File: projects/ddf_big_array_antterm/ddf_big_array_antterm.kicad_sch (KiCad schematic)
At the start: 11 parts, among them J1 Conn_Coaxial, J2 Conn_Coaxial

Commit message: release candidate
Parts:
- H1, H2, H3: now left out of the parts list
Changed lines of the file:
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@@
   )
   (symbol (lib_id "Mechanical:MountingHole_Pad") (at 48.006 170.434 0) (unit 1)
-    (in_bom yes) (on_board yes)
+    (in_bom no) (on_board yes)
     (property "Reference" "H1" (id 0) (at 50.546 169.1639 0)
       (effects (font (size 1.27 1.27)) (justify left))
@@
   )
   (symbol (lib_id "Mechanical:MountingHole_Pad") (at 65.151 170.434 0) (unit 1)
-    (in_bom yes) (on_board yes) (fields_autoplaced)
+    (in_bom no) (on_board yes) (fields_autoplaced)
     (property "Reference" "H2" (id 0) (at 67.691 169.1639 0)
       (effects (font (size 1.27 1.27)) (justify left))
@@
   )
   (symbol (lib_id "Mechanical:MountingHole_Pad") (at 82.296 170.434 0) (unit 1)
-    (in_bom yes) (on_board yes) (fields_autoplaced)
+    (in_bom no) (on_board yes) (fields_autoplaced)
     (property "Reference" "H3" (id 0) (at 84.836 169.1639 0)
       (effects (font (size 1.27 1.27)) (justify left))

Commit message: release candidate
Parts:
- H4: now left out of the parts list
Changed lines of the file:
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@@
   )
   (symbol (lib_id "Mechanical:MountingHole_Pad") (at 99.314 170.434 0) (unit 1)
-    (in_bom yes) (on_board yes) (fields_autoplaced)
+    (in_bom no) (on_board yes) (fields_autoplaced)
     (property "Reference" "H4" (id 0) (at 101.854 169.1639 0)
       (effects (font (size 1.27 1.27)) (justify left))

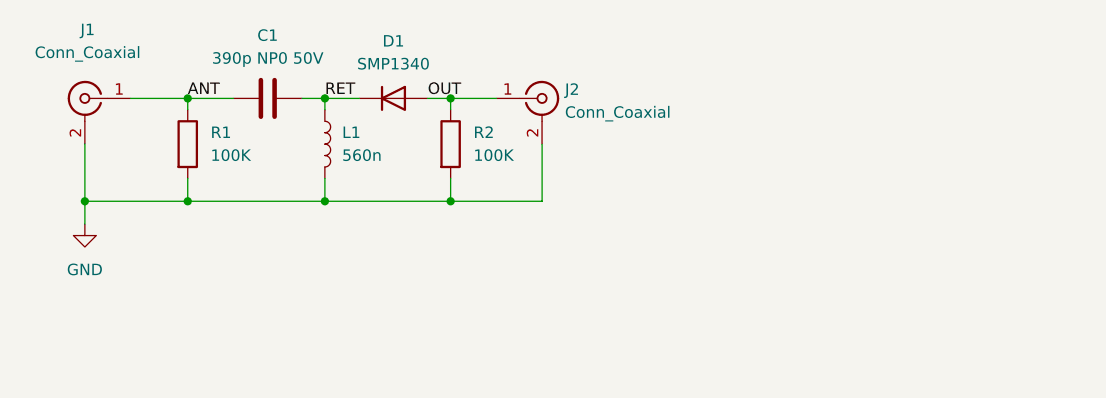
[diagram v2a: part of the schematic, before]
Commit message: release candidate
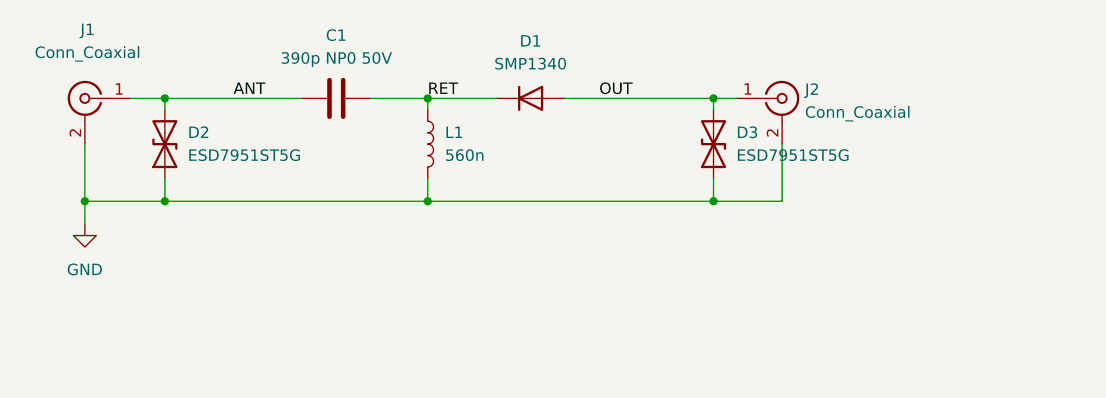
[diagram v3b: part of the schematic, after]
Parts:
- removed R1, R2: 100K, Resistor_SMD:R_0603_1608Metric, symbol Device:R
- added D2, D3: ESD7951ST5G, Diode_SMD:D_SOD-923, symbol Device:D_TVS
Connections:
- net ANT: now also D2.2 (A2)
- net GND: now also D2.1 (A1), D3.1 (A1)
- net OUT: now also D3.2 (A2)
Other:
- moved on the sheet: C1, D1, J2, L1

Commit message: release candidate
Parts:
- J1: LCSC (none) -> C2874833
- J2: LCSC (none) -> C1509208
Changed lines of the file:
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@@
       (effects (font (size 1.27 1.27)) hide)
     )
-    (property "Datasheet" "~" (id 3) (at 57.15 44.45 0)
+    (property "Datasheet" "https://www.onsemi.com/pdf/datasheet/esd7951s-d.pdf" (id 3) (at 57.15 44.45 0)
       (effects (font (size 1.27 1.27)) hide)
     )
@@
     )
     (property "Datasheet" " ~" (id 3) (at 125.73 39.37 0)
+      (effects (font (size 1.27 1.27)) hide)
+    )
+    (property "LCSC" "C1509208" (id 4) (at 125.73 39.37 0)
       (effects (font (size 1.27 1.27)) hide)
     )
@@
       (effects (font (size 1.27 1.27)) hide)
     )
+    (property "LCSC" "C2874833" (id 4) (at 48.26 39.37 0)
+      (effects (font (size 1.27 1.27)) hide)
+    )
     (pin "1")
     (pin "2")
@@
       (effects (font (size 1.27 1.27)) hide)
     )
-    (property "Datasheet" "~" (id 3) (at 118.11 44.45 0)
+    (property "Datasheet" "https://www.onsemi.com/pdf/datasheet/esd7951s-d.pdf" (id 3) (at 118.11 44.45 0)
       (effects (font (size 1.27 1.27)) hide)
     )
